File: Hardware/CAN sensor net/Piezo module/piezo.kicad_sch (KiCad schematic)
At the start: 13 parts, among them J4 532610271, U8 TL072, U9 ADS1120-PW

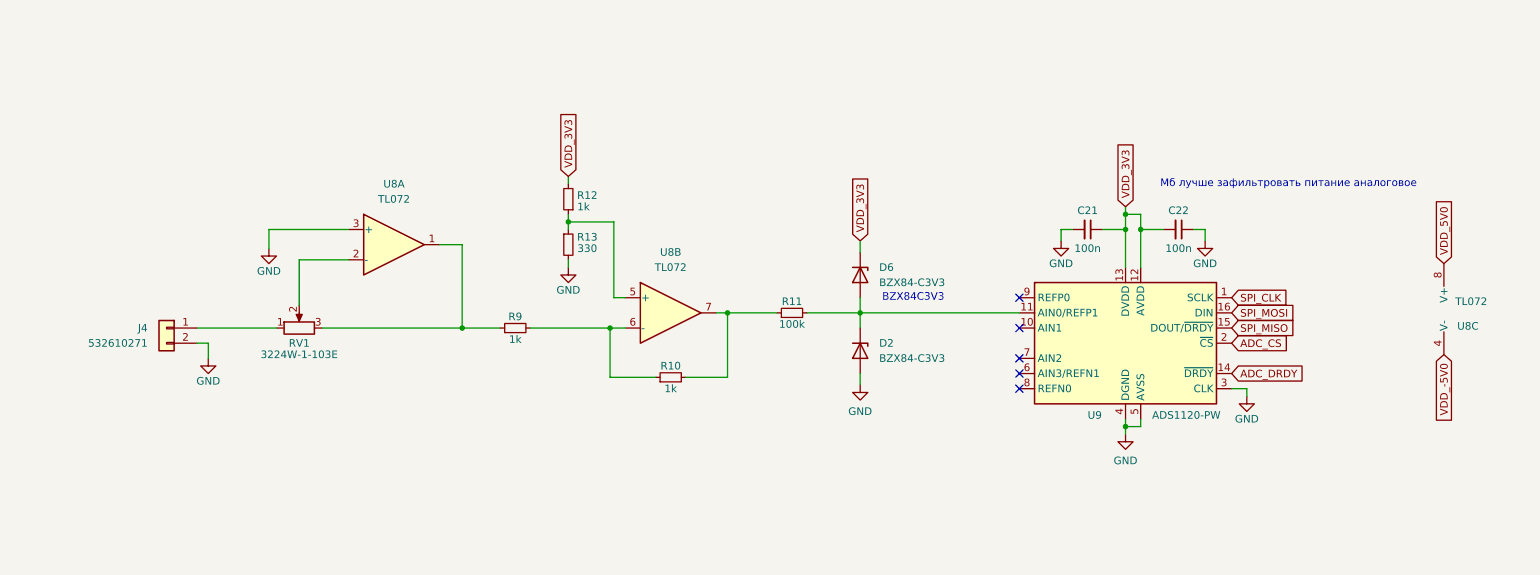
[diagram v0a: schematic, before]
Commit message: added band pass filter to piezo board
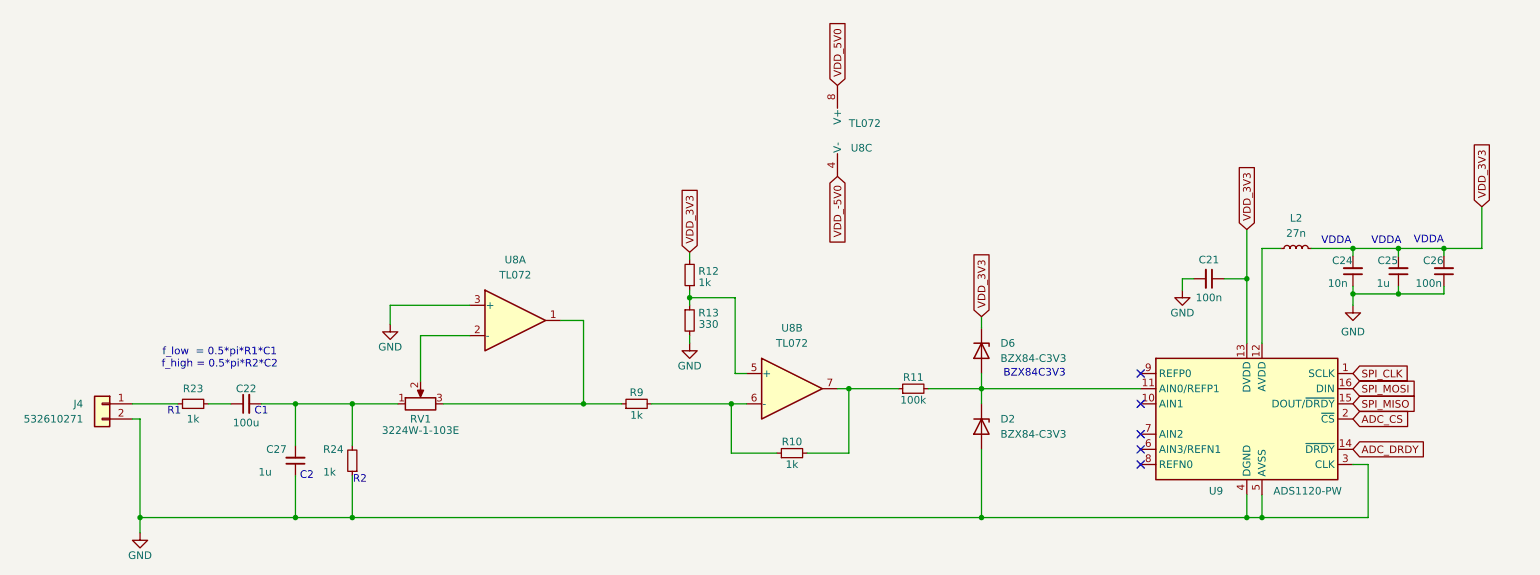
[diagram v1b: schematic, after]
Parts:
- added C24: 10n, Capacitor_SMD:C_0603_1608Metric, symbol Device:C_Small
- added C25: 1u, Capacitor_SMD:C_0603_1608Metric, symbol Device:C_Small
- added C26: 100n, Capacitor_SMD:C_0603_1608Metric, symbol Device:C_Small
- added C27: 1u, symbol Device:C_Small
- added L2: 27n, symbol Device:L_Small
- added R23, R24: 1k, symbol Device:R_Small
- C22: value 100n -> 100u; footprint Capacitor_SMD:C_0603_1608Metric -> (none)
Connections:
- net GND: now also C24.1, C25.1, C26.1, C27.1, R24.1; no longer C22.1
- net VDD_3V3: now also C24.2, C25.2, C26.2, L2.2; no longer C22.2, U9.12 (AVDD)
- net at RV1.1: now also C22.2, C27.2, R24.2; no longer J4.1 (Pin_1)
- new net: C22.1, R23.2
- new net: J4.1 (Pin_1), R23.1
- new net: L2.1, U9.12 (AVDD)
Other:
- note added: "C1"
- note added: "C2"
- note added: "R1"
- note added: "R2"
- note added: "VDDA"
- note added: "f_low = 0.5*pi*R1*C1 f_high = 0.5*pi*R2*C2"
- note removed: "Мб лучше зафильтровать питание аналоговое"
- moved on the sheet: C21, D2, D6, J4, R10, R11, R12, R13, R9, RV1, U8A, U8B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
